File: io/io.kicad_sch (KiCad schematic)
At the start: 4 parts, among them J2 AudioPlug4, J3 AudioPlug3, J4 AudioPlug3

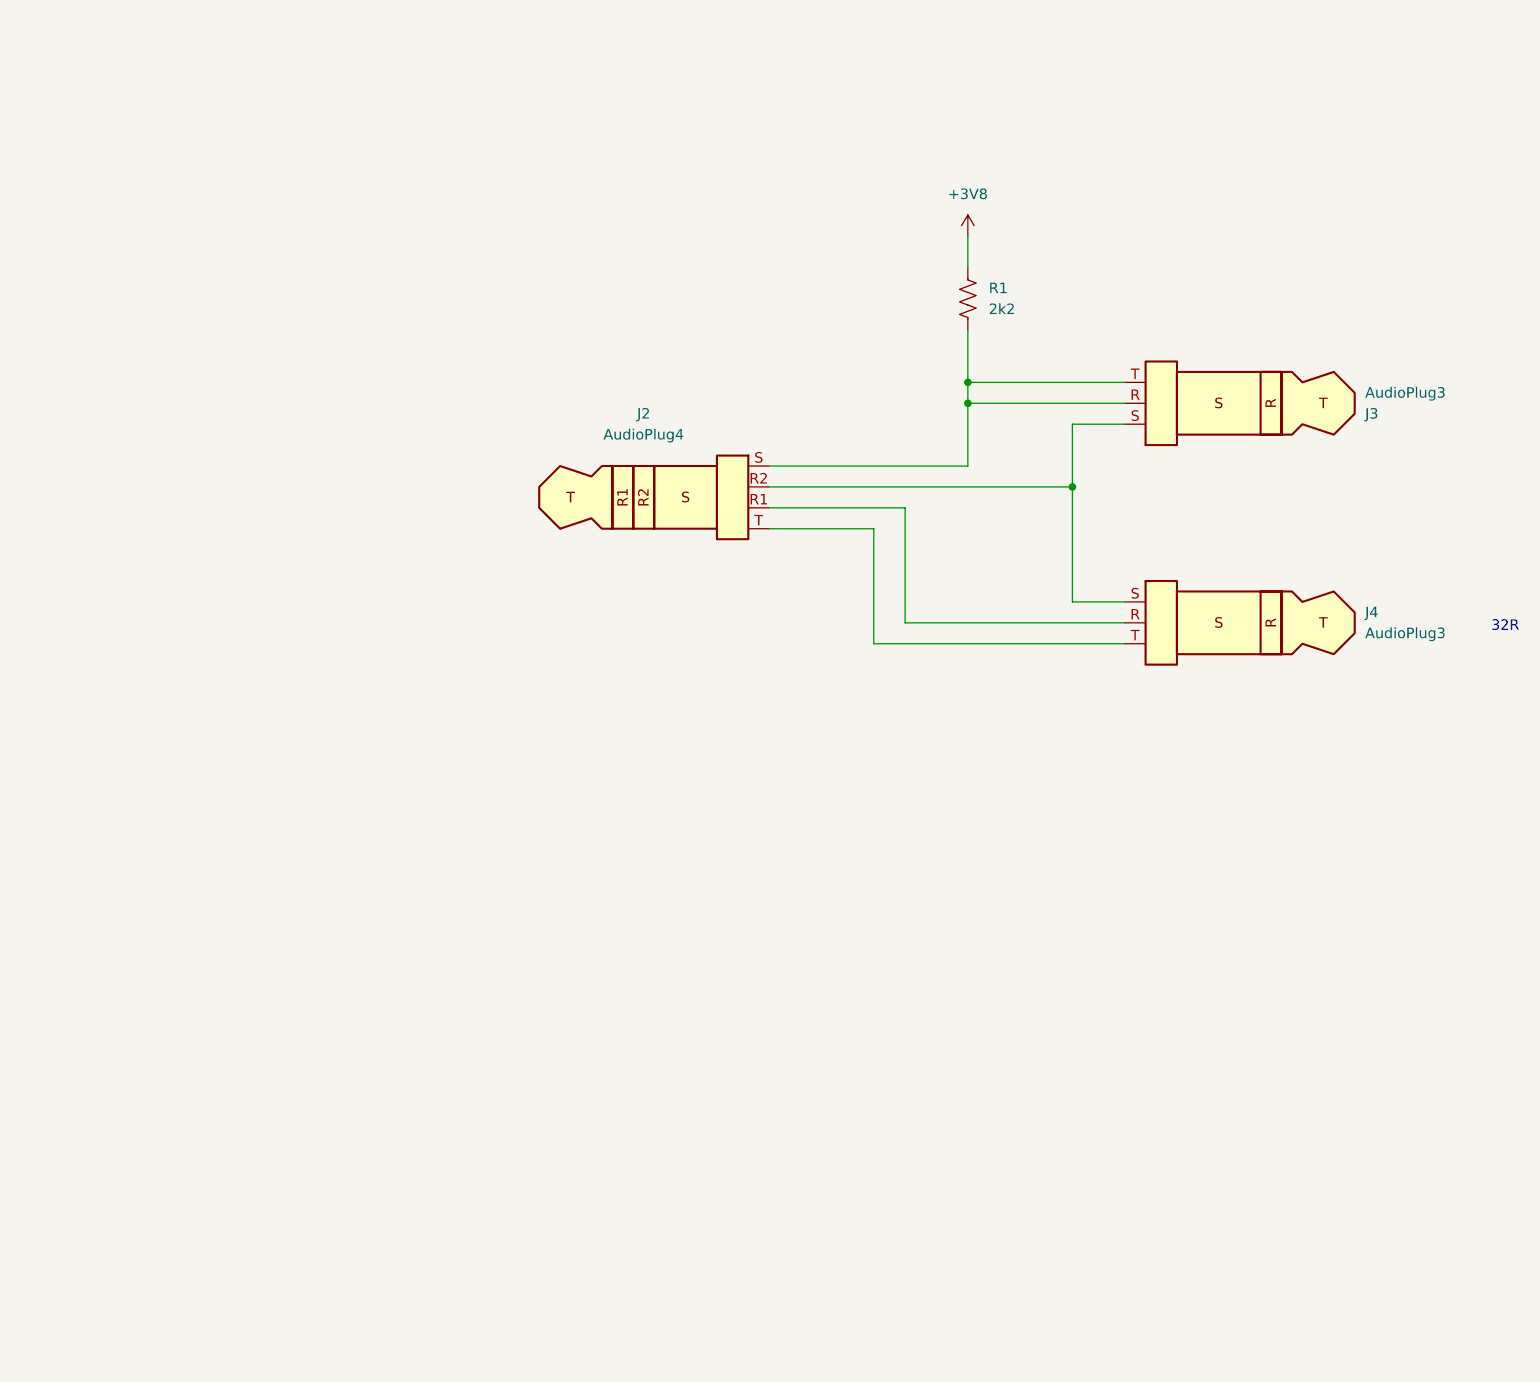
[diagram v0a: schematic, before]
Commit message: wip
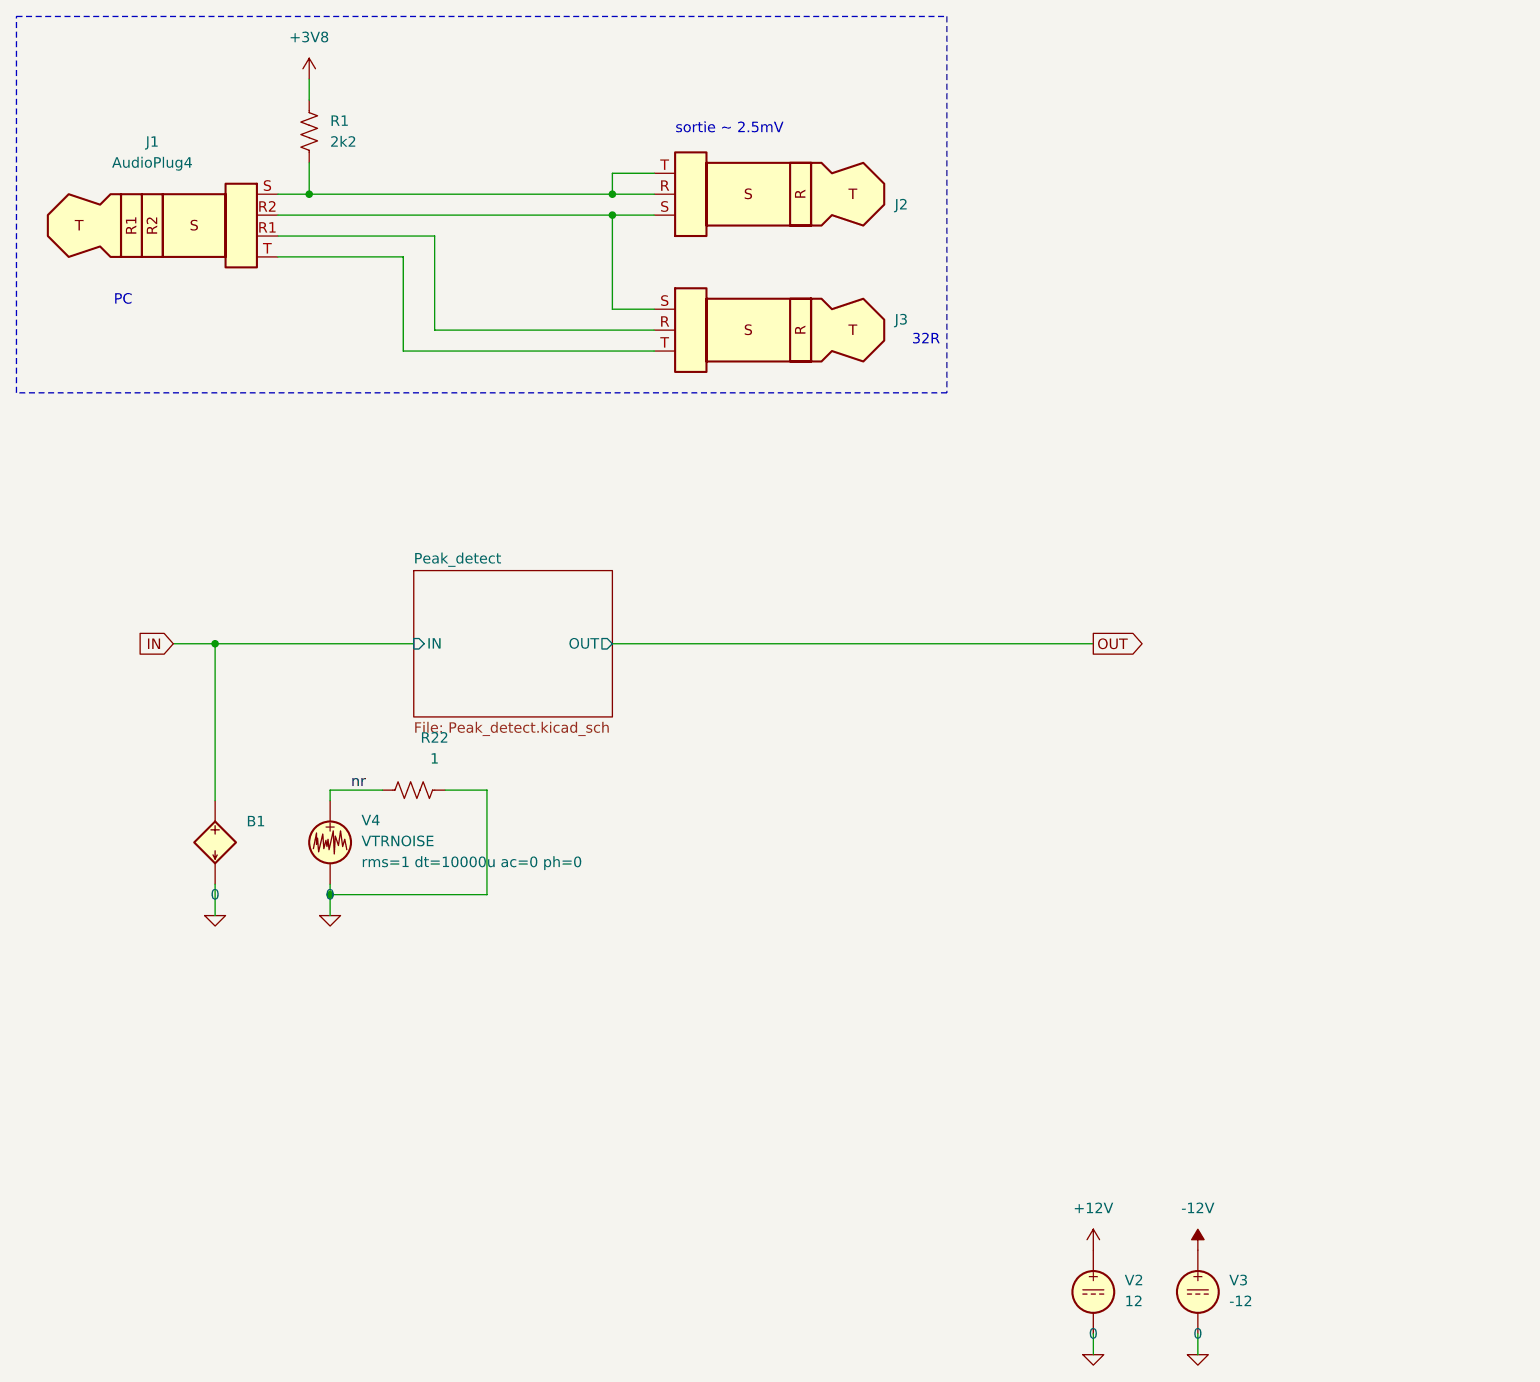
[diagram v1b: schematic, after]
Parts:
- added B1: BSOURCE, symbol Simulation_SPICE:BSOURCE
- added R22: 1, Resistor_THT:R_Axial_DIN0207_L6.3mm_D2.5mm_P10.16mm_Horizontal, symbol Device:R_US
- added V2: 12, symbol Simulation_SPICE:VDC
- added V3: -12, symbol Simulation_SPICE:VDC
- added V4: VTRNOISE, symbol Simulation_SPICE:VTRNOISE
- renumbered J2 to J1, J3 to J2, J4 to J3
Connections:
- new net +12V: V2.1
- new net -12V: V3.1
- new net 0: B1.2 (N-), R22.1, V2.2, V3.2, V4.2
- new net IN: B1.1 (N+)
- new net nr: R22.2, V4.1
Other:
- added sheet Peak_detect (Peak_detect.kicad_sch)
- note added: "PC"
- note added: "sortie ~ 2.5mV"
- moved on the sheet: J1, J2, J3, R1
